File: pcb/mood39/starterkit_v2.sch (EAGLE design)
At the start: 17 parts, among them IC1 TINY85, IC2 LM2940, X1 PWRUSB, X3 PWRUNREG

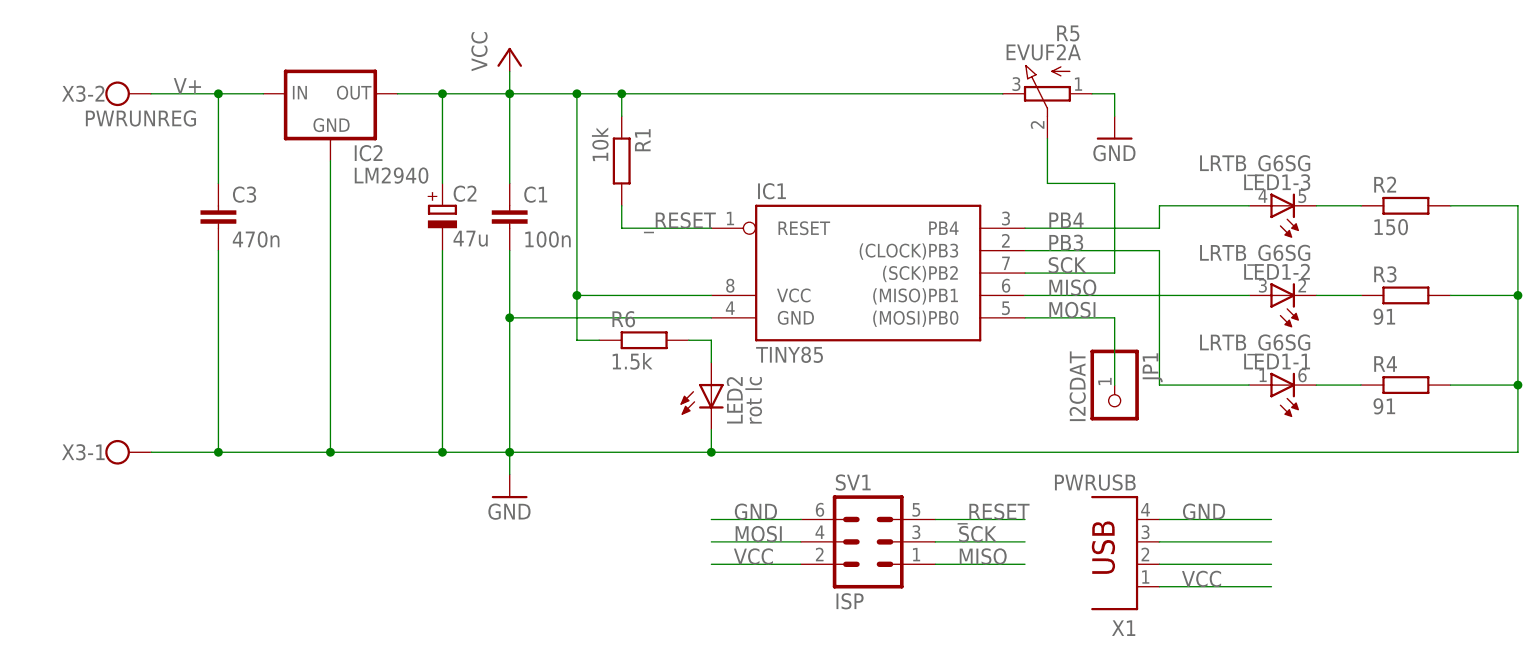
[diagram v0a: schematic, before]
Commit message: der miniaturtaster ist arg groß
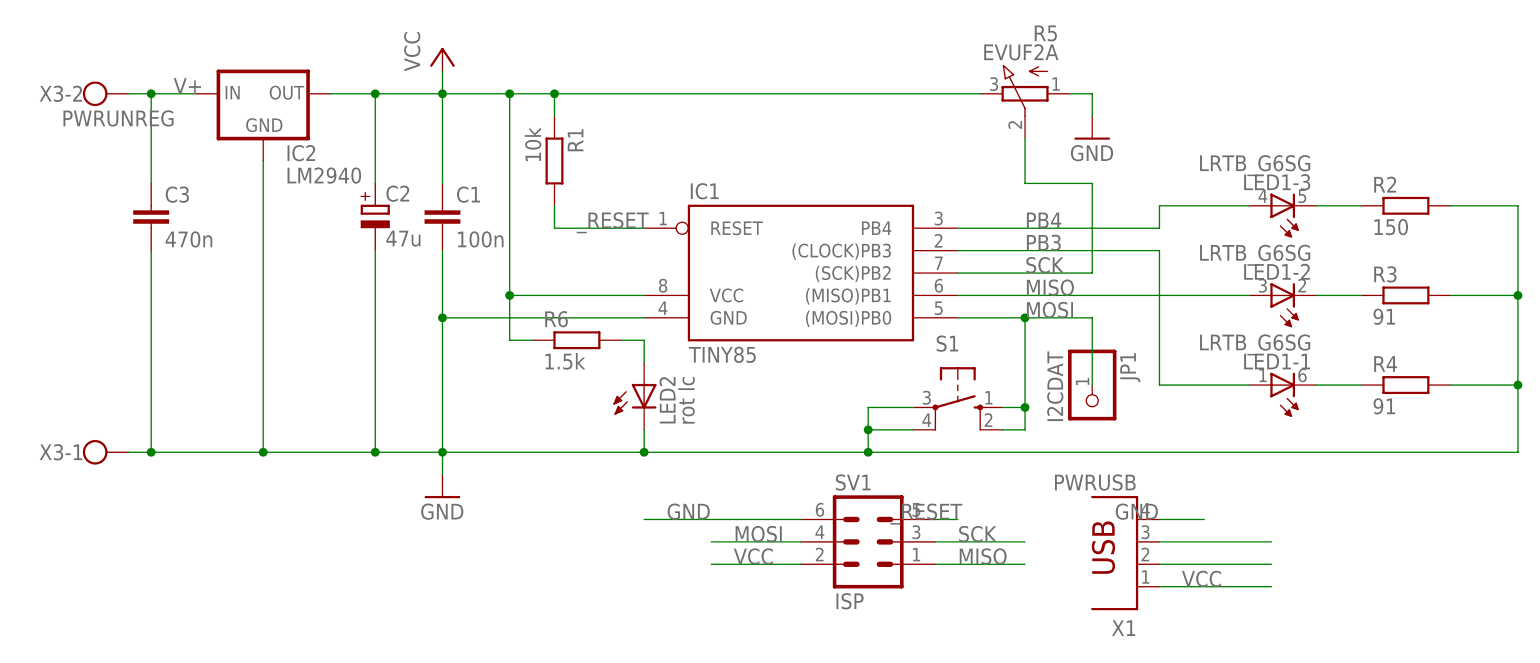
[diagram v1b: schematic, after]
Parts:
- added S1: (no value), switch-omron:10-XX
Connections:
- net GND: now also S1.P, S1.P1
- net MOSI: now also S1.S, S1.S1
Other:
- moved on the sheet: C1, C2, C3, IC1, IC2, JP1, LED2, R1, R5, R6, X3-1, X3-2
